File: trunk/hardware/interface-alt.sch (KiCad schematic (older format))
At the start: 19 parts, among them SW1 DIPSW4_DIP, U4 GTL2003

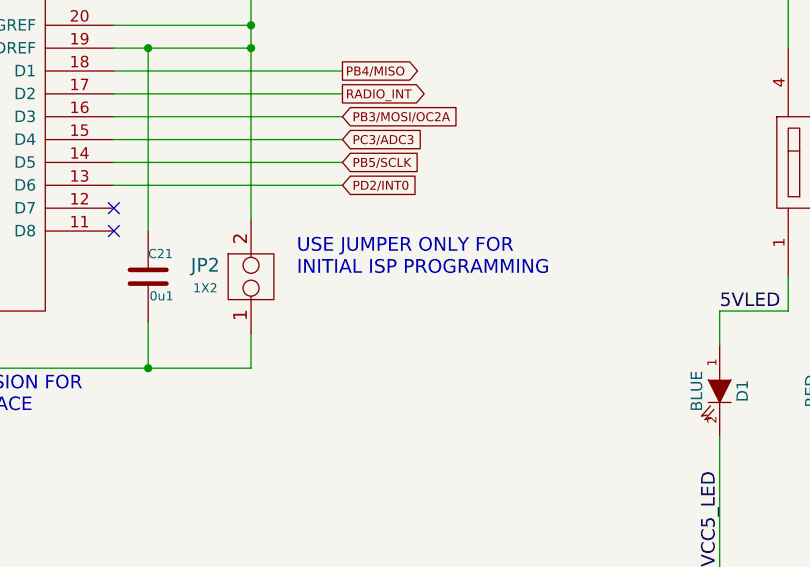
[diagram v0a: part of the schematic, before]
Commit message: Final tidy-ups for (hopefully) final PCB fabrication. Bumped version to v1.2.
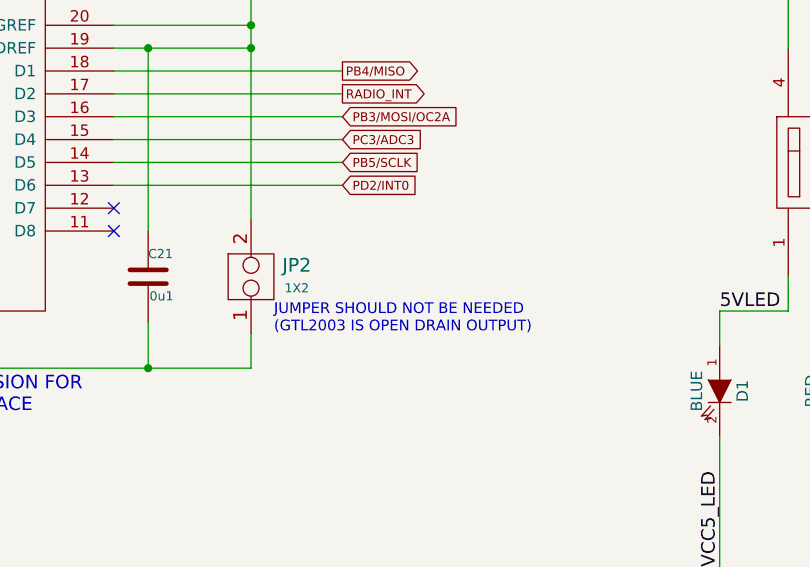
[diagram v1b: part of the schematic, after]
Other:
- note added: "JUMPER SHOULD NOT BE NEEDED\n(GTL2003 IS OPEN DRAIN OUTPUT)"
- note removed: "USE JUMPER ONLY FOR\nINITIAL ISP PROGRAMMING"
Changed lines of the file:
@@
 Title "FREAKDUINO-CHIBI 2.4GHz"
 Date "16 aug 2013"
-Rev "v1.1"
+Rev "v1.2"
 Comp "KiCAD version by Gruvin"
 Comment1 ""
@@
 U 1 1 51E3DC42
 P 4400 3700
-F 0 "JP2" H 4200 3750 60  0000 C CNN
-F 1 "1X2" H 4200 3650 40  0000 C CNN
+F 0 "JP2" H 4600 3750 60  0000 C CNN
+F 1 "1X2" H 4600 3650 40  0000 C CNN
 F 2 "" H 4400 3700 60  0000 C CNN
 F 3 "" H 4400 3700 60  0000 C CNN
@@
 	1    0    0    -1
 $EndComp
-Text Notes 4600 3700 0    60   ~ 0
-USE JUMPER ONLY FOR\nINITIAL ISP PROGRAMMING
+Text Notes 4500 3950 0    47   ~ 0
+JUMPER SHOULD NOT BE NEEDED\n(GTL2003 IS OPEN DRAIN OUTPUT)
 $Comp
 L DIPSW4_DIP SW1
